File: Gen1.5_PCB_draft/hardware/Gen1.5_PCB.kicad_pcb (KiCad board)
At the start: 4 copper layers, 74.8 x 101.5 mm, 67 parts, among them IC1 TJA1050T, J1 Enc1, J10 jumper2, J11 jumper4, J12 Enc2, J13 Enc3, J14 Enc4, J15 Enc5, J16 Enc6, J17 UART/CAN, J2 Booster, J4 UART/CAN, J5 MCP1, J6 MCP2, J7 MCP3, J8 UART/CAN, J9 jumper5, P2 LC1, P3 LC2, P4 LC3, P5 LC4, U1 ESP32-P4-ETH, U10 INA118U_2K5, U11 INA118U_2K5, U12 INA118U_2K5, U2 4754, U4 REF2033QDDCRQ1, U8 level shifter, U9 INA118U_2K5

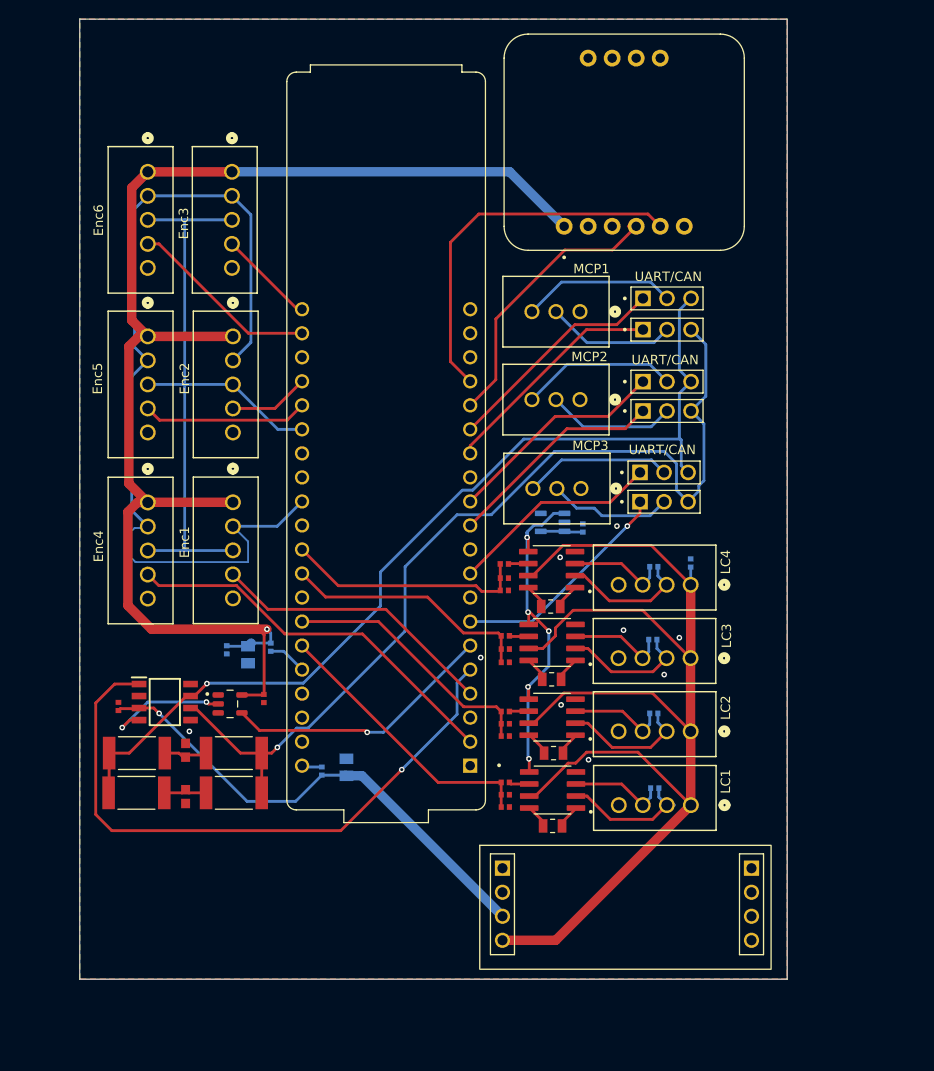
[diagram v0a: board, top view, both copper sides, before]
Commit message: fixed pcb
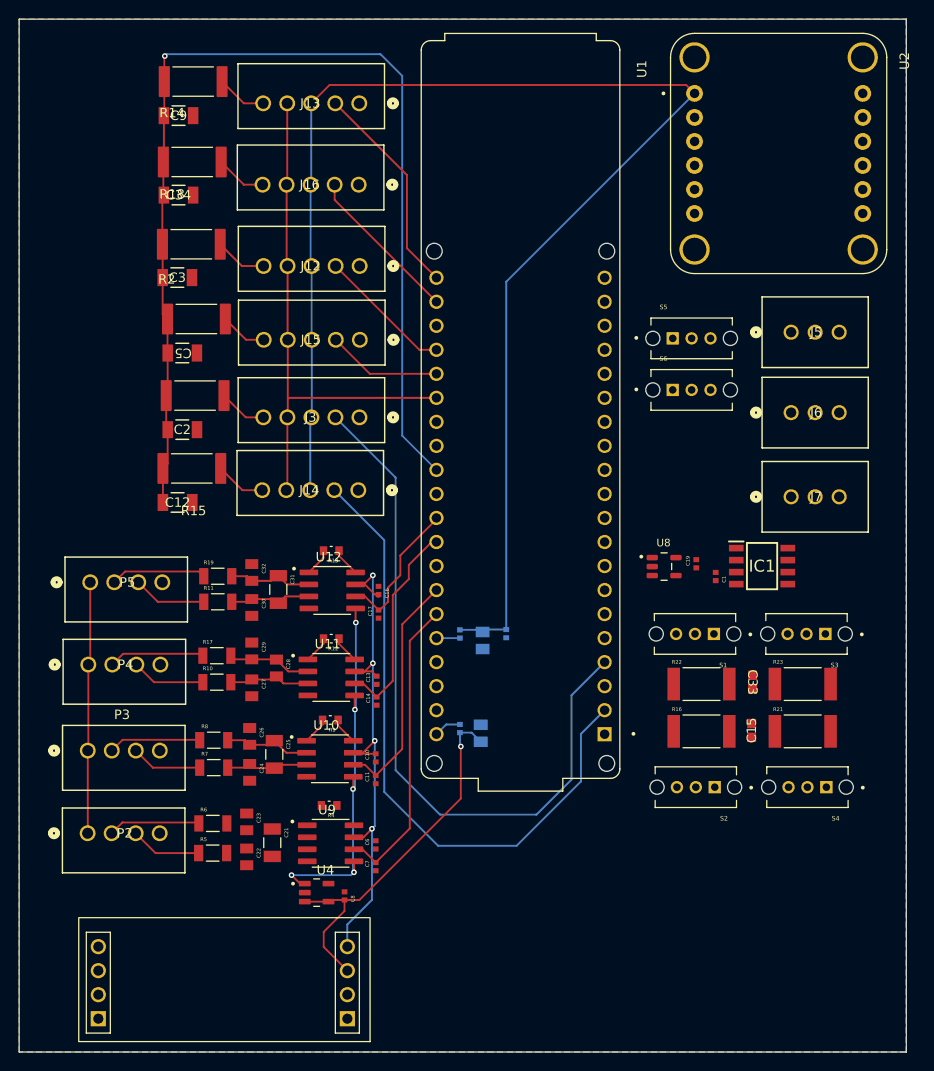
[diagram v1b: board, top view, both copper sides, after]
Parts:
- removed J1: Enc1, Gen1.5_PCB:molex_5pin
- removed J10: jumper2, Gen1.5_PCB:CONN_3pin_jumper
- removed J11: jumper4, Gen1.5_PCB:CONN_3pin_jumper
- removed J17, J4, J8: UART/CAN, Gen1.5_PCB:CONN_3pin_jumper
- removed J9: jumper5, Gen1.5_PCB:CONN_3pin_jumper
- added C21: 68nF, Gen1.5_PCB:CAP_68nF, F.Cu at (140.5, 115.7)
- added C22: 6.8nF, Gen1.5_PCB:CAP_6.8nF, F.Cu at (137.8, 117.2)
- added C23: 6.8nF, Gen1.5_PCB:CAP_6.8nF, F.Cu at (137.8, 113.5)
- added C24: 6.8nF, Gen1.5_PCB:CAP_6.8nF, F.Cu at (138.1, 108.2)
- added C25: 68nF, Gen1.5_PCB:CAP_68nF, F.Cu at (140.7, 106.3)
- added C26: 6.8nF, Gen1.5_PCB:CAP_6.8nF, F.Cu at (138.1, 104.4)
- added C27: 6.8nF, Gen1.5_PCB:CAP_6.8nF, F.Cu at (138.3, 99.3)
- added C28: 68nF, Gen1.5_PCB:CAP_6.8nF, F.Cu at (140.9, 97.2)
- added C29: 6.8nF, Gen1.5_PCB:CAP_6.8nF, F.Cu at (138.3, 95.4)
- added C30: 6.8nF, Gen1.5_PCB:CAP_6.8nF, F.Cu at (138.3, 90.8)
- added C31: 68nF, Gen1.5_PCB:CAP_68nF, F.Cu at (141.1, 88.9)
- added C32: 6.8nF, Gen1.5_PCB:CAP_6.8nF, F.Cu at (138.3, 87.1)
- added C33: 47nF, Gen1.5_PCB:CAP_47nF, F.Cu at (191.2, 98.7)
- added C34: 8.2nF, Gen1.5_PCB:CAP_8.2nF, F.Cu at (130.6, 47.2)
- added J3: Enc1, Gen1.5_PCB:molex_5pin, F.Cu at (149.7, 70.7)
- added R17: 5k, Gen1.5_PCB:RES_5k, F.Cu at (134.6, 95.9)
- added R18: 10, Gen1.5_PCB:RES_10, F.Cu at (132.0, 43.7)
- added R19: 5k, Gen1.5_PCB:RES_5k, F.Cu at (134.7, 87.5)
- added R21: 60, Gen1.5_PCB:RES_60, F.Cu at (196.5, 103.9)
- added R22: 60, Gen1.5_PCB:RES_60, F.Cu at (185.8, 98.9)
- added R23: 60, Gen1.5_PCB:RES_60, F.Cu at (196.5, 98.9)
- added S1: EN termination low, Gen1.5_PCB:switch, F.Cu at (185.2, 93.6)
- added S2: EN loopback low, Gen1.5_PCB:switch, F.Cu at (185.2, 109.8)
- added S3: EN termination high, Gen1.5_PCB:switch, F.Cu at (196.9, 93.6)
- added S4: EN loopback high, Gen1.5_PCB:switch, F.Cu at (197.0, 109.8)
- added S5: jumper1, Gen1.5_PCB:switch, F.Cu at (184.8, 62.4)
- added S6: jumper2, Gen1.5_PCB:switch, F.Cu at (184.8, 67.8)
- C10, C13, C16, C6, C8, U4: moved to F.Cu
- C12, C5, C9: value 0.1uf -> 8.2nF; footprint Gen1.5_PCB:CAP_0.1uF_50V -> Gen1.5_PCB:CAP_8.2nF; moved to F.Cu
- C15: value 0.1uf -> 47nF; footprint Gen1.5_PCB:CAP_0.1uF_50V -> Gen1.5_PCB:CAP_47nF; moved to F.Cu
- C2, C3: value 47nF -> 8.2nF; footprint Gen1.5_PCB:CAP_47nF -> Gen1.5_PCB:CAP_8.2nF
- J5: value MCP1 -> Roboclaw1
- J6: value MCP2 -> Roboclaw2
- J7: value MCP3 -> Roboclaw3
- P2: value LC1 -> loadcell 1
- P3: value LC2 -> loadcell 2
- P4: value LC3 -> loadcell 3
- P5: value LC4 -> loadcell 4
- R1, R2, R3: value 60 -> 10; footprint Gen1.5_PCB:RES_60 -> Gen1.5_PCB:RES_10
- R10, R7: value 500 -> 5k; footprint Gen1.5_PCB:RES_510 -> Gen1.5_PCB:RES_5k
- R11, R5, R8: value 33k -> 5k; footprint Gen1.5_PCB:RES_33k -> Gen1.5_PCB:RES_5k
- R12, R9: value 12k -> 931; footprint Gen1.5_PCB:RES_12k -> Gen1.5_PCB:RES_931
- R13, R4: value 500 -> 931; footprint Gen1.5_PCB:RES_510 -> Gen1.5_PCB:RES_931
- R14: value 33k -> 10; footprint Gen1.5_PCB:RES_33k -> Gen1.5_PCB:RES_10
- R15: value 12k -> 10; footprint Gen1.5_PCB:RES_12k -> Gen1.5_PCB:RES_10
- R6: value 12k -> 5k; footprint Gen1.5_PCB:RES_12k -> Gen1.5_PCB:RES_5k
- moved C9 80.7 mm to (130.6, 38.8), turned to 0 degrees
- moved C5 67.9 mm to (130.9, 63.9), turned to 0 degrees
- moved IC1 64.8 mm to (192.2, 86.4)
- moved C1 64.6 mm to (187.3, 87.5), turned to -90 degrees
- moved P2 63.8 mm to (120.9, 114.7), turned to 180 degrees
- moved P3 63.8 mm to (121.0, 105.9), turned to 180 degrees
- moved P4 63.7 mm to (121.0, 96.8), turned to 180 degrees
- moved P5 63.5 mm to (121.2, 88.1), turned to 180 degrees
- moved R14 60.7 mm to (132.1, 35.2)
- moved R2 58.2 mm to (131.9, 52.4), turned to 180 degrees
- moved C12 52.3 mm to (130.5, 79.7), turned to 0 degrees
- moved C3 50.0 mm to (130.4, 55.9), turned to 0 degrees
- moved R16 49.5 mm to (185.8, 103.9)
- moved U8 48.1 mm to (181.9, 86.5)
- moved C19 47.9 mm to (185.3, 86.2)
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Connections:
- C1 pad 1: /5V -> 5V
- C12 pad 1: /loadcells/Vin(-) 3 -> /MISO
- C12 pad 2: /loadcells/Vin(+) 3 -> GND
- C15 pad 1: /loadcells/Vin(-) 4 -> Net-(C15-Pad1)
- C15 pad 2: /loadcells/Vin(+) 4 -> GND
- C2 pad 1: GND -> /MISO
- C2 pad 2: Net-(C2-Pad2) -> GND
- C20 pad 1: /5V -> 5V
- C3 pad 1: GND -> /MISO
- C3 pad 2: Net-(C3-Pad2) -> GND
- C5 pad 1: /loadcells/Vin(-) 1 -> /MISO
- C5 pad 2: /loadcells/Vin(+) 1 -> GND
- C8 pad 2: /loadcells/5V -> 5V
- C9 pad 1: /loadcells/Vin(-) 2 -> /MISO
- C9 pad 2: /loadcells/Vin(+) 2 -> GND
- FB2 pad 1: /5V -> 5V
- IC1 pad 3: /5V -> 5V
- J12 pad 1: /3V3 -> GND
- J12 pad 2: /MISO -> /CS2
- J12 pad 3: /CLK -> /3V3
- J12 pad 4: /CS2 -> /CLK
- J12 pad 5: GND -> Net-(J12-Pin_5)
- J13 pad 1: /3V3 -> GND
- J13 pad 2: /MISO -> /CS4
- J13 pad 3: /CLK -> /3V3
- J13 pad 4: /CS4 -> /CLK
- J13 pad 5: GND -> Net-(J13-Pin_5)
- J14 pad 1: /3V3 -> GND
- J14 pad 2: /MISO -> /CS6
- J14 pad 3: /CLK -> /3V3
- J14 pad 4: /CS6 -> /CLK
- J14 pad 5: GND -> Net-(J14-Pin_5)
- J15 pad 1: /3V3 -> GND
- J15 pad 2: /MISO -> /CS1
- J15 pad 3: /CLK -> /3V3
- J15 pad 4: /CS1 -> /CLK
- J15 pad 5: GND -> Net-(J15-Pin_5)
- J16 pad 1: /3V3 -> GND
- J16 pad 2: /MISO -> /CS3
- J16 pad 3: /CLK -> /3V3
- J16 pad 4: /CS3 -> /CLK
- J16 pad 5: GND -> Net-(J16-Pin_5)
- J2 pad 3: /5V -> 5V
- J6 pad 2: Net-(J11-Pin_2) -> /TX2
- J6 pad 3: Net-(J6-Pin_3) -> /RX2
- J7 pad 2: Net-(J17-Pin_2) -> /TX3
- J7 pad 3: Net-(J7-Pin_3) -> /RX3
- R1 pad 1: /CANH -> Net-(J3-Pin_5)
- R1 pad 2: Net-(C2-Pad2) -> /MISO
- R10 pad 1: Net-(U11-RG__1) -> /loadcells/Vin(+) 3
- R10 pad 2: Net-(U11-RG) -> Net-(U11-V+_IN)
- R11 pad 1: /loadcells/INAout 3 -> /loadcells/Vin(+) 4
- R11 pad 2: LC3 -> Net-(U12-V+_IN)
- R12 pad 1: GND -> Net-(U11-RG__1)
- R12 pad 2: LC3 -> Net-(U11-RG)
- R14 pad 1: /loadcells/INAout 4 -> Net-(J13-Pin_5)
- R14 pad 2: LC4 -> /MISO
- R15 pad 1: GND -> Net-(J14-Pin_5)
- R15 pad 2: LC4 -> /MISO
- R16 pad 1: Net-(C3-Pad2) -> /LL
- R16 pad 2: /CANL -> Net-(C15-Pad1)
- R2 pad 1: Net-(C2-Pad2) -> Net-(J12-Pin_5)
- R2 pad 2: /CANL -> /MISO
- R3 pad 1: /CANH -> Net-(J15-Pin_5)
- R3 pad 2: Net-(C3-Pad2) -> /MISO
- R5 pad 1: /loadcells/INAout 1 -> /loadcells/Vin(+) 1
- R5 pad 2: LC1 -> Net-(U9-V+_IN)
- R6 pad 1: GND -> /loadcells/Vin(-) 1
- R6 pad 2: LC1 -> Net-(U9-V-_IN)
- R7 pad 1: Net-(U10-RG__1) -> /loadcells/Vin(+) 2
- R7 pad 2: Net-(U10-RG) -> Net-(U10-V+_IN)
- R8 pad 1: /loadcells/INAout 2 -> /loadcells/Vin(-) 2
- R8 pad 2: LC2 -> Net-(U10-V-_IN)
- R9 pad 1: GND -> Net-(U10-RG__1)
- R9 pad 2: LC2 -> Net-(U10-RG)
- U10 pad 2: /loadcells/Vin(-) 2 -> Net-(U10-V-_IN)
- U10 pad 3: /loadcells/Vin(+) 2 -> Net-(U10-V+_IN)
- U10 pad 6: /loadcells/INAout 2 -> LC2
- U11 pad 2: /loadcells/Vin(-) 3 -> Net-(U11-V-_IN)
- U11 pad 3: /loadcells/Vin(+) 3 -> Net-(U11-V+_IN)
- U11 pad 6: /loadcells/INAout 3 -> LC3
- U12 pad 2: /loadcells/Vin(-) 4 -> Net-(U12-V-_IN)
- U12 pad 3: /loadcells/Vin(+) 4 -> Net-(U12-V+_IN)
- U12 pad 6: /loadcells/INAout 4 -> LC4
- U4 pad 3: /loadcells/5V -> 5V
- U4 pad 4: /loadcells/5V -> 5V
- U9 pad 2: /loadcells/Vin(-) 1 -> Net-(U9-V-_IN)
- U9 pad 3: /loadcells/Vin(+) 1 -> Net-(U9-V+_IN)
- U9 pad 6: /loadcells/INAout 1 -> LC1
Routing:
- net /CANL: track 101.1 -> 0.00 mm, vias 1 -> 0
- net /CANH: track 100.9 -> 0.00 mm, vias 1 -> 0
- net /CAN TX: track 66.5 -> 0.00 mm, vias 1 -> 0
- net 10V: track 140.5 -> 85.1 mm, vias 0 -> 4
- net /5V: track 51.6 -> 0.00 mm, vias 1 -> 0
- net /CS5: track 30.3 -> 75.9 mm
- net 5V: track 0.00 -> 40.0 mm, vias 0 -> 1
- net /SDA: track 39.5 -> 0.00 mm
- net /SCL: track 30.0 -> 0.00 mm
- net /CAN RX_1: track 28.8 -> 0.00 mm, vias 1 -> 0
- net /CS6: track 41.4 -> 68.6 mm
- net /TX1: track 24.2 -> 0.00 mm
- net /RX1: track 24.0 -> 0.00 mm
- net /TX3: track 23.9 -> 0.00 mm, vias 1 -> 0
- net /RX2: track 23.5 -> 0.00 mm
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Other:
- board size 74.8 x 101.5 mm -> 93.8 x 109.2 mm
